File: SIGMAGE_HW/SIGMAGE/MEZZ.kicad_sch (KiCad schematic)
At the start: 4 parts, among them J12 61306421821, J13 61306421121, J14 61306421821, J8 61306421121

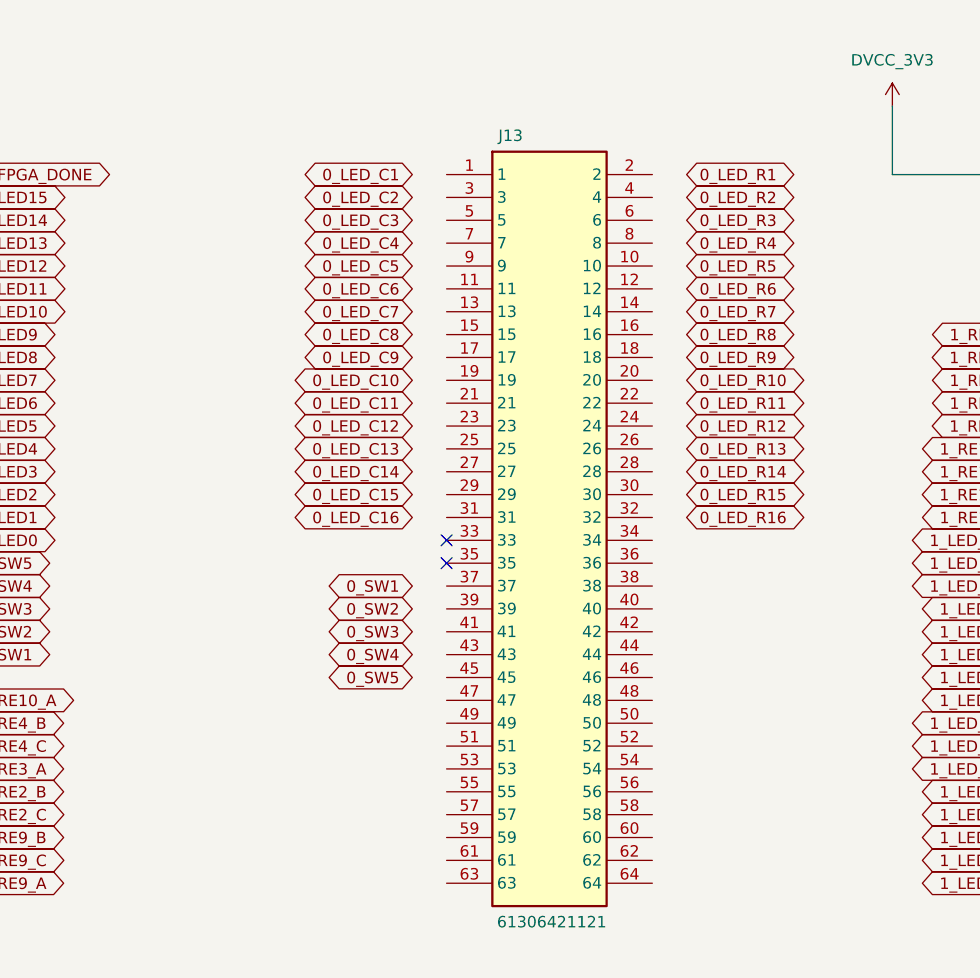
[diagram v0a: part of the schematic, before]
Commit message: some foo
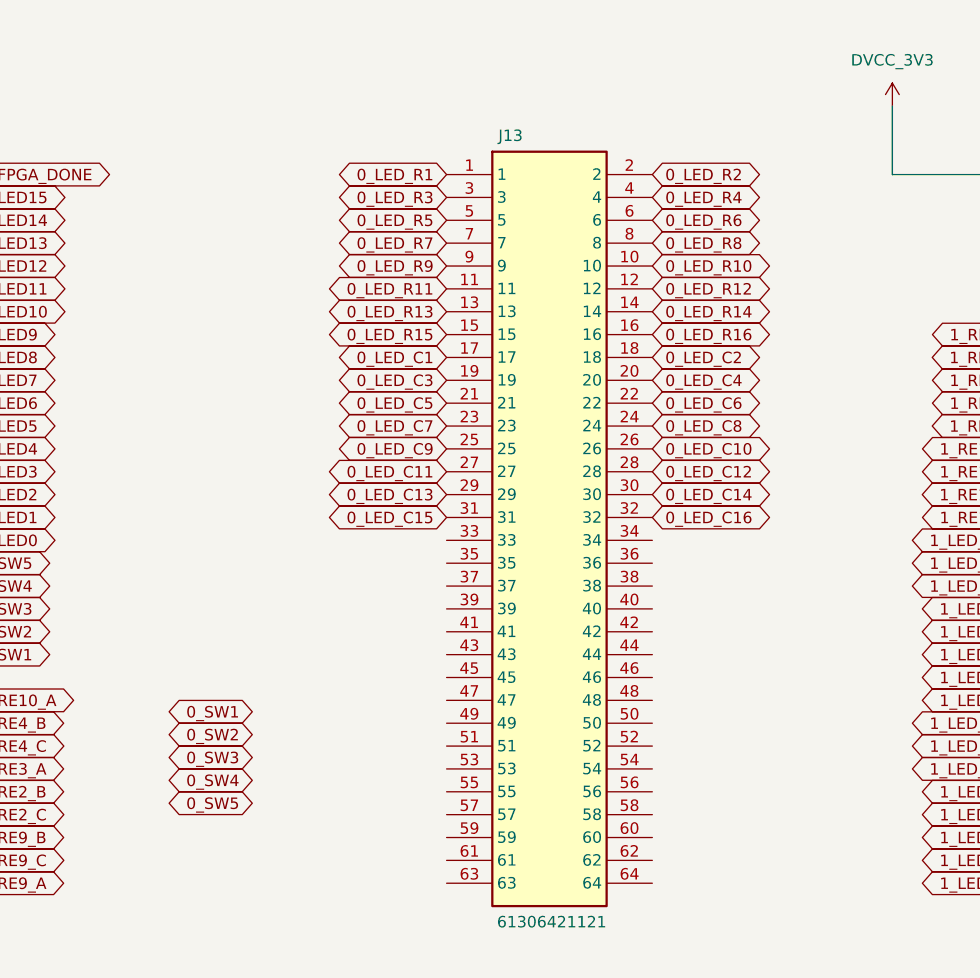
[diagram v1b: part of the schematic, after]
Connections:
- net 0_LED_C1: now also J13.17
- net 0_LED_C10: now also J13.26
- net 0_LED_C11: now also J13.27
- net 0_LED_C12: now also J13.28
- net 0_LED_C13: now also J13.29
- net 0_LED_C14: now also J13.30
- net 0_LED_C15: now also J13.31
- net 0_LED_C16: now also J13.32
- net 0_LED_C2: now also J13.18
- net 0_LED_C3: now also J13.19
- net 0_LED_C4: now also J13.20
- net 0_LED_C5: now also J13.21
- net 0_LED_C6: now also J13.22
- net 0_LED_C7: now also J13.23
- net 0_LED_C8: now also J13.24
- net 0_LED_C9: now also J13.25
- net 0_LED_R1: now also J13.1
- net 0_LED_R10: now also J13.10
- net 0_LED_R11: now also J13.11
- net 0_LED_R12: now also J13.12
- net 0_LED_R13: now also J13.13
- net 0_LED_R14: now also J13.14
- net 0_LED_R15: now also J13.15
- net 0_LED_R16: now also J13.16
- net 0_LED_R2: now also J13.2
- net 0_LED_R3: now also J13.3
- net 0_LED_R4: now also J13.4
- net 0_LED_R5: now also J13.5
- net 0_LED_R6: now also J13.6
- net 0_LED_R7: now also J13.7
- net 0_LED_R8: now also J13.8
- net 0_LED_R9: now also J13.9
- no-connect marks 3 -> 1
